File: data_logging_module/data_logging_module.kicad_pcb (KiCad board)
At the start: 2 copper layers, 77.5 x 45 mm, 60 parts, among them J1 Conn_01x15, J2 Conn_01x15, J200 10067847-001RLF, U100 TLV62569DBV, U101 HT7533-1, U300 BME280, U301 BME280, U400 PCF8563TS, U5 DS18B20, Y400 32768Hz

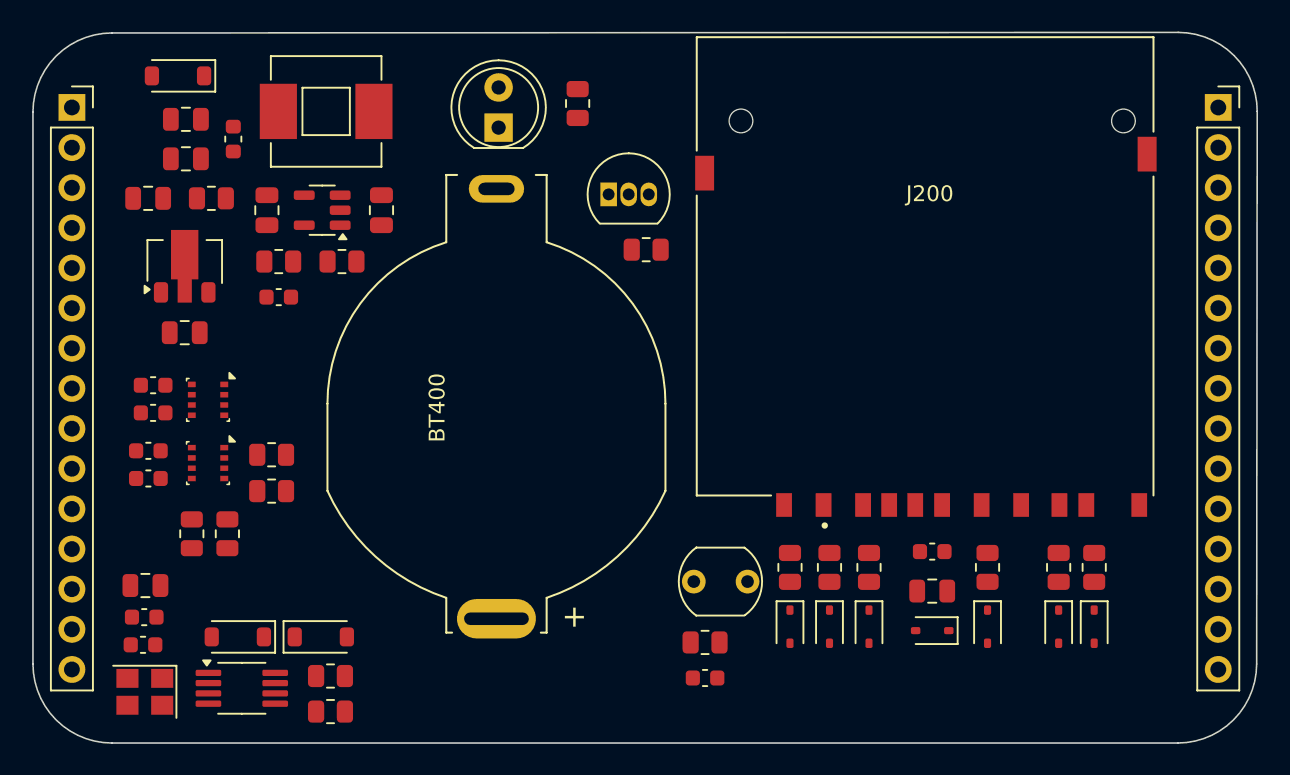
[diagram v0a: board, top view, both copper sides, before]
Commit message: initial PCB
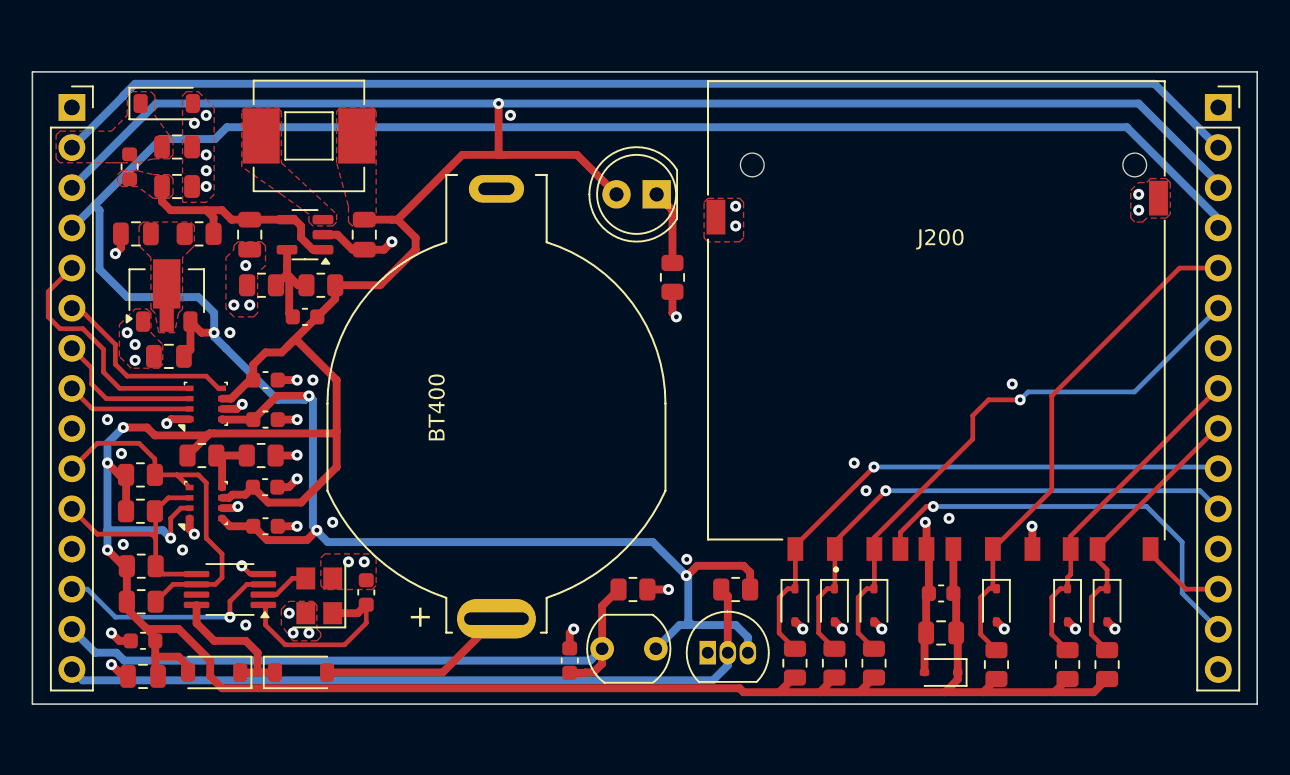
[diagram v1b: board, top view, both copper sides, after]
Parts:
- moved U5 29.7 mm to (115.2, 84.2)
- moved R301 22.2 mm to (117.0, 80.2)
- moved R400 15.1 mm to (79.4, 78.8), turned to 0 degrees
- moved C402 14.5 mm to (93.6, 80.4), turned to 90 degrees
- moved R401 12.9 mm to (79.4, 81.0), turned to 0 degrees
- moved Y400 12.6 mm to (90.7, 80.7), turned to 90 degrees
- moved R106 12.5 mm to (113.0, 60.5), turned to 90 degrees
- moved D101 10.9 mm to (112.0, 55.2), turned to 180 degrees
- moved R302 9.04 mm to (79.3, 75.3), turned to 0 degrees
- moved C302 8.82 mm to (87.2, 76.2), turned to 0 degrees
- moved C300 8.63 mm to (106.5, 84.8), turned to 90 degrees
- moved R303 8.36 mm to (79.3, 73.0), turned to 0 degrees
- moved C304 7.44 mm to (87.2, 69.5), turned to 0 degrees
- moved C303 7.41 mm to (87.2, 67.0), turned to 0 degrees
- moved C301 7.41 mm to (87.2, 73.8), turned to 0 degrees
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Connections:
- J1 pad 13: LDR -> PCF8563_INT
- J1 pad 14: DS18B20 -> LDR
- J1 pad 15: PCF8563_INT -> DS18B20
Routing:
- net +3.3V: track 0.00 -> 263.8 mm, vias 0 -> 5
- net +3.3VA: track 0.00 -> 167.2 mm, vias 0 -> 4
- net VIN: track 0.00 -> 75.9 mm
- net DS18B20: track 0.00 -> 47.2 mm
- net GND: track 0.00 -> 42.3 mm, vias 0 -> 59
- net LDR: track 0.00 -> 42.1 mm
- net SD_CARD_CMD/MOSI: track 0.00 -> 36.8 mm, vias 0 -> 1
- net SD_CARD_DAT2: track 0.00 -> 36.5 mm, vias 0 -> 1
- net SD_CARD_CS/DAT3: track 0.00 -> 34.0 mm, vias 0 -> 1
- net SD_CARD_CLK/SCK: track 0.00 -> 32.7 mm
- net SD_CARD_CD: track 0.00 -> 27.0 mm, vias 0 -> 1
- net I2C_SCL: track 0.00 -> 23.2 mm
- net SD_CARD_DAT0/MISO: track 0.00 -> 21.6 mm
- net SD_CARD_DAT1: track 0.00 -> 18.6 mm
- net BME280_SCK: track 0.00 -> 15.4 mm
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- added copper zone on F.Cu, net +3.3V
- added copper zone on F.Cu, net +5V
- added copper zone on F.Cu, net /[1]Power/+5V_FILT
- added copper zone on F.Cu, net /[1]Power/BUCK_SW
- added copper zone on F.Cu, net GND
- added copper zone on In1.Cu, net GND
- added copper zone on In2.Cu, net GND
- added copper zone on F.Cu, net VIN
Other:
- board size 77.5 x 45 mm -> 77.5 x 40 mm
- copper layers 2 -> 4
